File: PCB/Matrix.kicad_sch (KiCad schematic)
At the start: 132 parts, among them Q1 MMFTN620KD, Q2 MMFTN620KD, Q3 MMFTN620KD, Q4 MMFTN620KD

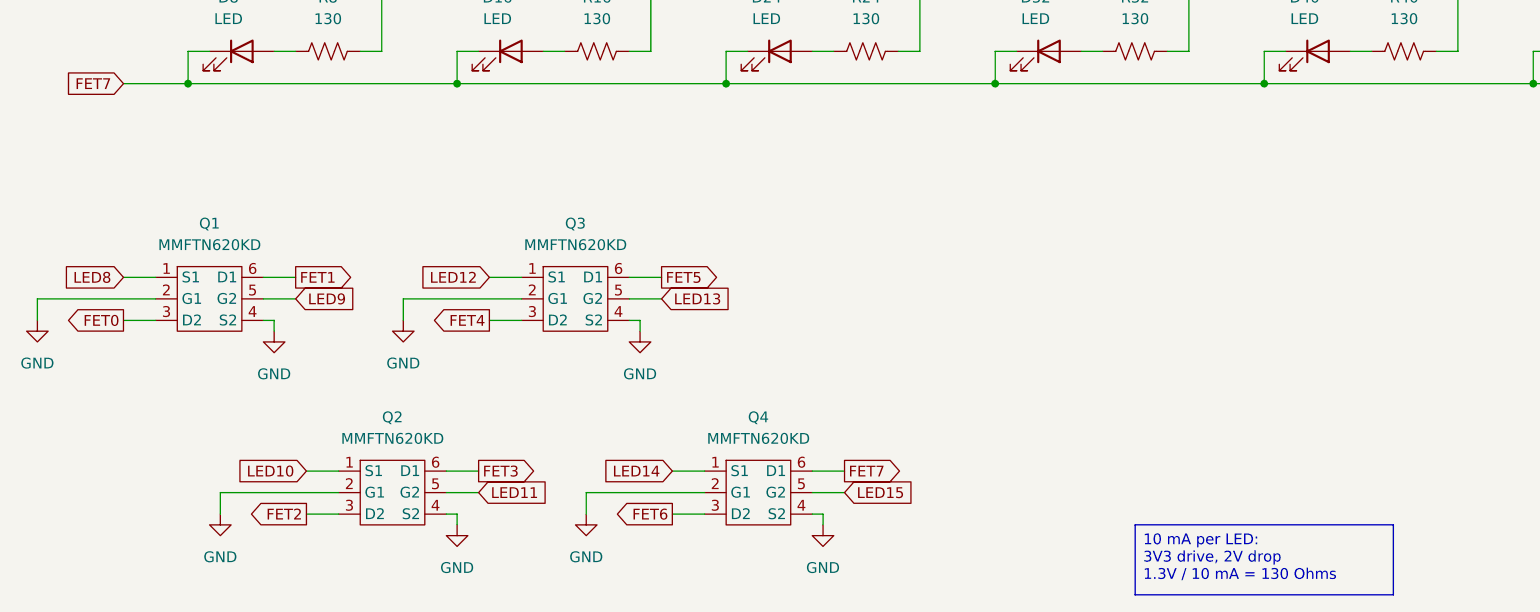
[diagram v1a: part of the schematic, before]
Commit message: Fixed Q1-Q4, re-released
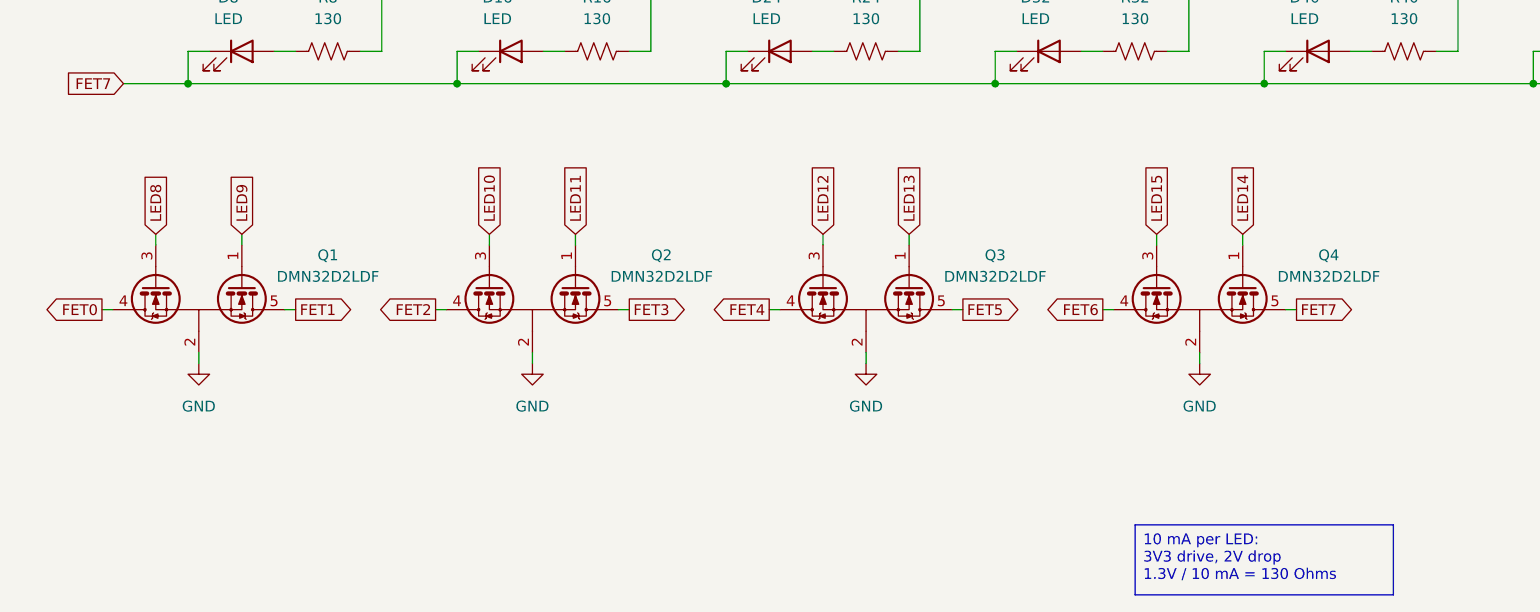
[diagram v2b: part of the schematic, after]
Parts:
- removed Q1, Q2, Q3, Q4: MMFTN620KD, Package_TO_SOT_SMD:SOT-457T, symbol VolumetricDisplay:MMFTN620KD
- added Q1, Q2, Q3, Q4: DMN32D2LDF, Package_TO_SOT_SMD:SOT-353_SC-70-5, symbol Transistor_FET:DMN32D2LDF
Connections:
- net FET0: now also Q1.4 (D2)
- net FET1: now also Q1.5 (D1)
- net FET2: now also Q2.4 (D2)
- net FET3: now also Q2.5 (D1)
- net FET4: now also Q3.4 (D2)
- net FET5: now also Q3.5 (D1)
- net FET6: now also Q4.4 (D2)
- net FET7: now also Q4.5 (D1)
- net GND: now also Q1.2 (S), Q2.2 (S), Q3.2 (S), Q4.2 (S)
- net LED10: now also Q2.3 (G2)
- net LED11: now also Q2.1 (G1)
- net LED12: now also Q3.3 (G2)
- net LED13: now also Q3.1 (G1)
- net LED14: now also Q4.1 (G1)
- net LED15: now also Q4.3 (G2)
- net LED8: now also Q1.3 (G2)
- net LED9: now also Q1.1 (G1)
